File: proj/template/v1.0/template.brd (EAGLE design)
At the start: 40.6 x 21.6 mm, 1 part

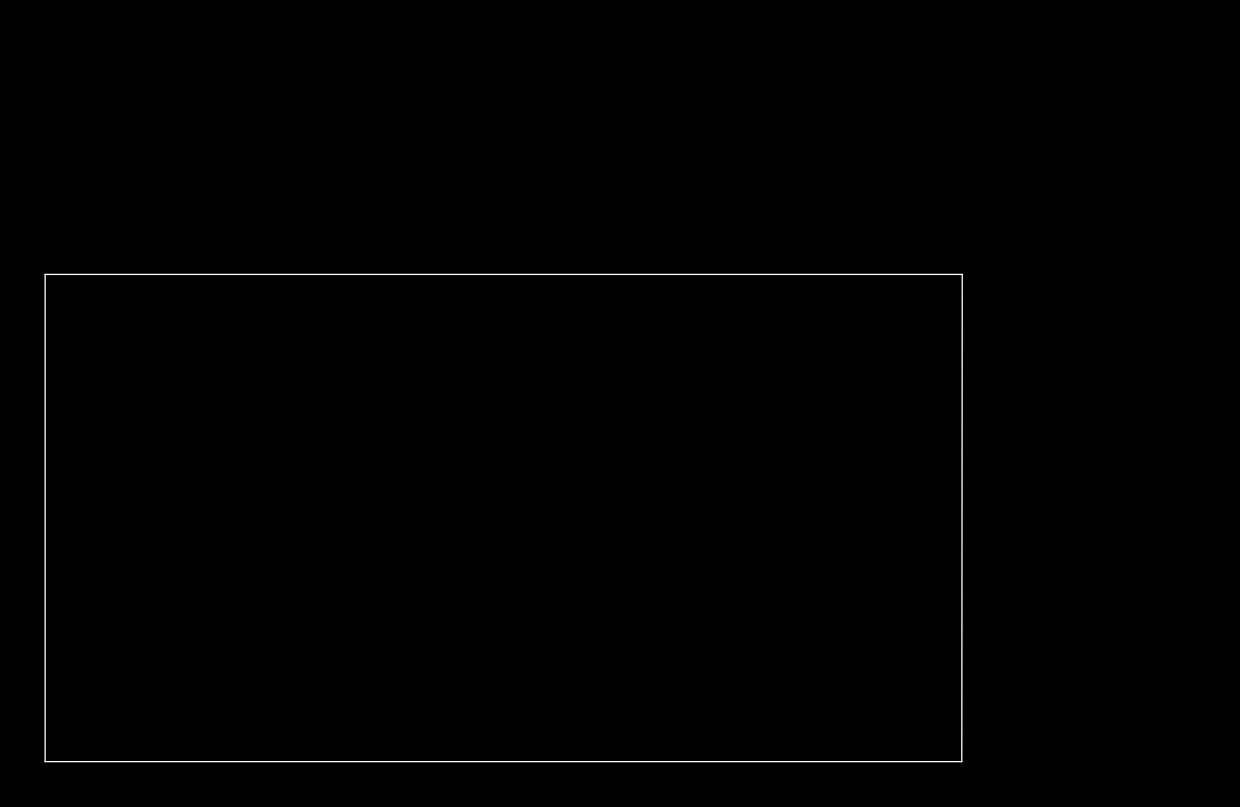
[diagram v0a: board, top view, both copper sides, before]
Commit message: pushing to avoid any loss of work
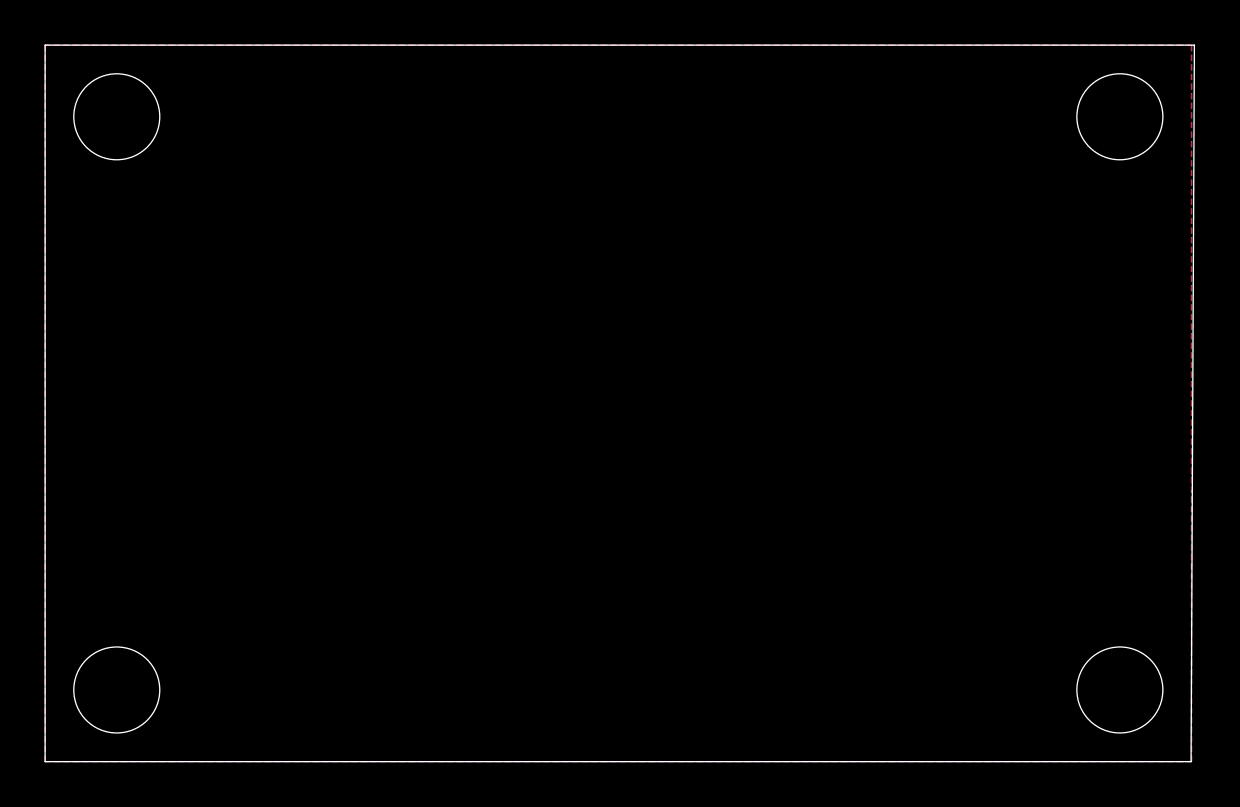
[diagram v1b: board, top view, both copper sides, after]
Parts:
- moved FRAME1 7.18 mm to (44.5, 6.35)
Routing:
- added copper zone on layer 1, net GND
- added copper zone on layer 16, net GND
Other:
- board size 40.6 x 21.6 mm -> 50.9 x 31.8 mm
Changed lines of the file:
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@@
 <?xml version="1.0" encoding="utf-8"?>
 <!DOCTYPE eagle SYSTEM "eagle.dtd">
-<eagle version="8.4.2">
+<eagle version="8.4.3">
 <drawing>
 <settings>
@@
 <setting verticaltext="up"/>
 </settings>
-<grid distance="50" unitdist="mil" unit="mil" style="lines" multiple="1" display="yes" altdistance="5" altunitdist="mil" altunit="mil"/>
+<grid distance="125" unitdist="mil" unit="mil" style="lines" multiple="1" display="yes" altdistance="5" altunitdist="mil" altunit="mil"/>
 <layers>
 <layer number="1" name="Top" color="4" fill="1" visible="yes" active="yes"/>
@@
 <layer number="43" name="vRestrict" color="2" fill="10" visible="yes" active="yes"/>
 <layer number="44" name="Drills" color="7" fill="1" visible="no" active="yes"/>
-<layer number="45" name="Holes" color="7" fill="1" visible="no" active="yes"/>
+<layer number="45" name="Holes" color="7" fill="1" visible="yes" active="yes"/>
 <layer number="46" name="Milling" color="3" fill="1" visible="no" active="yes"/>
 <layer number="47" name="Measures" color="7" fill="1" visible="no" active="yes"/>
@@
 <board>
 <plain>
-<wire x1="0" y1="0" x2="40.62" y2="0" width="0" layer="20"/>
-<wire x1="40.62" y1="0" x2="40.64" y2="21.59" width="0" layer="20"/>
-<wire x1="40.64" y1="21.59" x2="0" y2="21.59" width="0" layer="20"/>
-<wire x1="0" y1="21.59" x2="0" y2="0" width="0" layer="20"/>
+<wire x1="0" y1="0" x2="50.78" y2="0" width="0" layer="20"/>
+<wire x1="50.78" y1="0" x2="50.927" y2="31.75" width="0" layer="20"/>
+<wire x1="50.927" y1="31.75" x2="0" y2="31.75" width="0" layer="20"/>
+<wire x1="0" y1="31.75" x2="0" y2="0" width="0" layer="20"/>
+<hole x="3.175" y="3.175" drill="3.81"/>
+<hole x="47.625" y="3.175" drill="3.81"/>
+<hole x="3.175" y="28.575" drill="3.81"/>
+<hole x="47.625" y="28.575" drill="3.81"/>
 </plain>
 <attributes>
@@
 </autorouter>
 <elements>
-<element name="FRAME1" library="openag-frames" package="DOCFIELD" value="" x="39.37" y="1.27" rot="MR0">
-<attribute name="AUTHOR" value="XX" x="39.37" y="1.27" size="1.778" layer="28" rot="MR0" display="off"/>
-<attribute name="DESCRIPTION" value="Template for starting new designs." x="39.37" y="1.27" size="1.778" layer="28" rot="MR0" display="off"/>
-<attribute name="TITLE" value="Example Template!" x="39.37" y="1.27" size="1.778" layer="28" rot="MR0" display="off"/>
-<attribute name="URL" value="https://github.com/OpenAgInitiative/openag_eagle_template" x="39.37" y="1.27" size="1.778" layer="28" rot="MR0" display="off"/>
-<attribute name="VER" value="1.0" x="39.37" y="1.27" size="1.778" layer="28" rot="MR0" display="off"/>
+<element name="FRAME1" library="openag-frames" package="DOCFIELD" value="" x="44.45" y="6.35" rot="MR0">
+<attribute name="AUTHOR" value="XX" x="44.45" y="6.35" size="1.778" layer="28" rot="MR0" display="off"/>
+<attribute name="DESCRIPTION" value="Template for starting new designs." x="44.45" y="6.35" size="1.778" layer="28" rot="MR0" display="off"/>
+<attribute name="TITLE" value="Example Template!" x="44.45" y="6.35" size="1.778" layer="28" rot="MR0" display="off"/>
+<attribute name="URL" value="https://github.com/OpenAgInitiative/openag_eagle_template" x="44.45" y="6.35" size="1.778" layer="28" rot="MR0" display="off"/>
+<attribute name="VER" value="1.0" x="44.45" y="6.35" size="1.778" layer="28" rot="MR0" display="off"/>
 </element>
 </elements>
 <signals>
+<signal name="GND">
+<polygon width="0.3048" layer="1" isolate="0.4064" rank="3">
+<vertex x="0" y="0"/>
+<vertex x="50.8" y="0"/>
+<vertex x="50.8" y="31.75"/>
+<vertex x="0" y="31.75"/>
+</polygon>
+<polygon width="0.3048" layer="16" isolate="0.4064" rank="3">
+<vertex x="0" y="31.75"/>
+<vertex x="50.8" y="31.75"/>
+<vertex x="50.8" y="0"/>
+<vertex x="0" y="0"/>
+</polygon>
+</signal>
 </signals>
 </board>
